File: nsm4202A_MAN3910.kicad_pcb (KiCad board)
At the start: 2 copper layers, 40.5 x 25.5 mm, 19 parts, among them IC1 IS31FL3730-QFLS2-TR, IC2 IS31FL3730-QFLS2-TR, J1 Conn_01x07_Pin, J2 Conn_01x02_Pin, J3 Conn_01x03_Pin

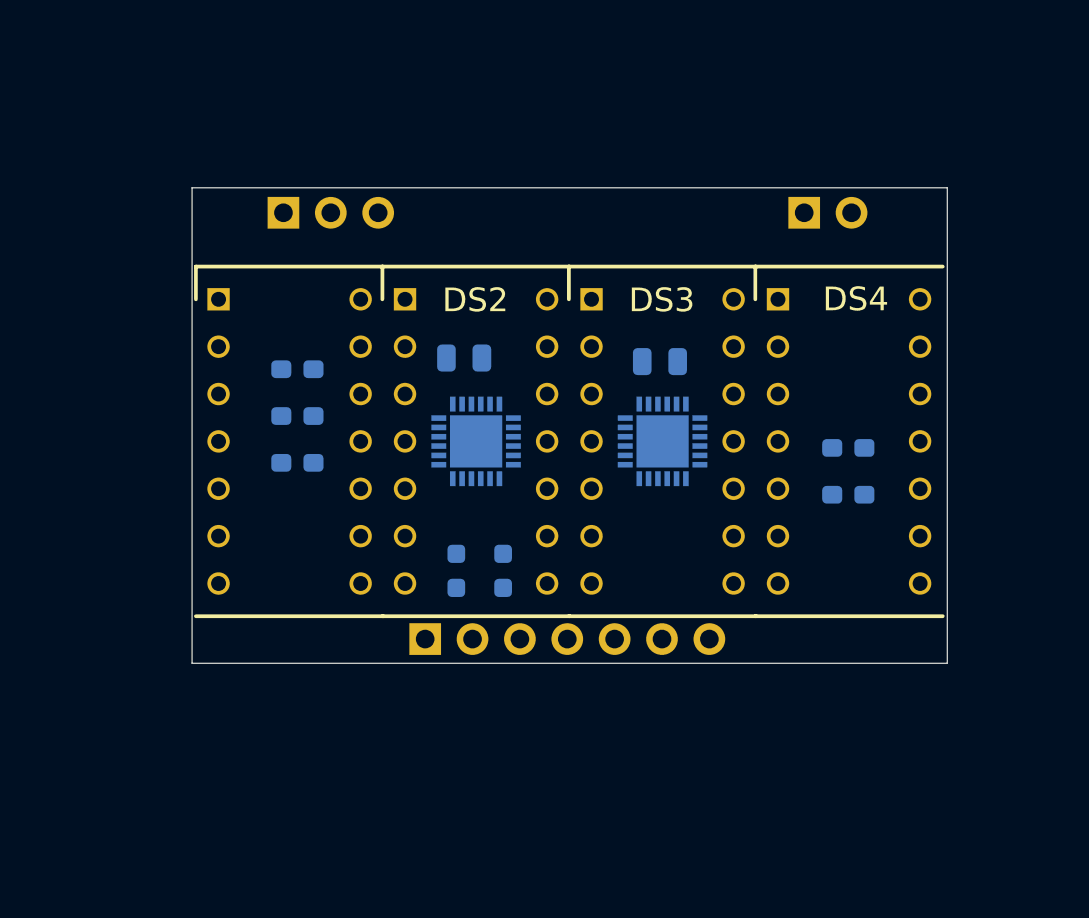
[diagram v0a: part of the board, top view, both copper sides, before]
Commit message: Start trace
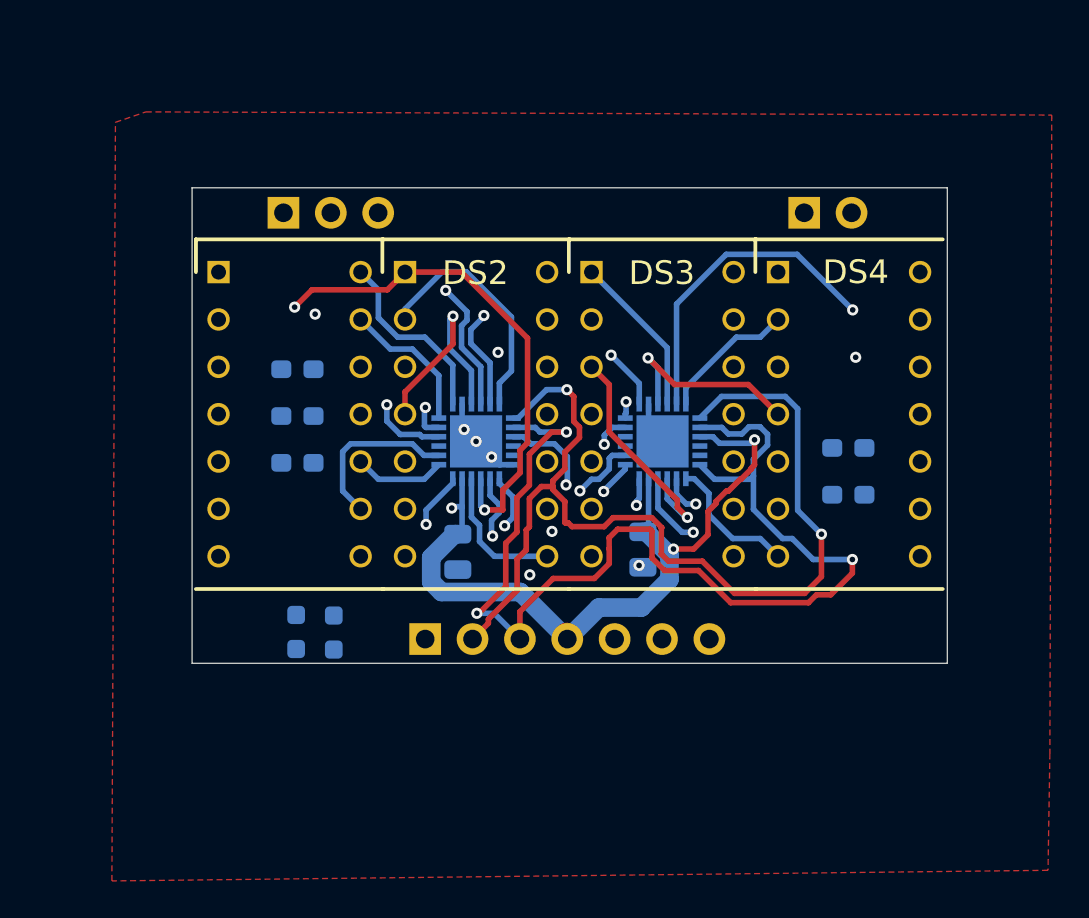
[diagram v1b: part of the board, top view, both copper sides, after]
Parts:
- moved R2 11.6 mm to (105.6, 98.8)
- moved C3 10.4 mm to (114.2, 94.5), turned to -90 degrees
- moved C7 10.1 mm to (124.2, 94.4), turned to -90 degrees
- moved R1 7.36 mm to (107.6, 98.8)
- moved DS1 1.46 mm to (101.4, 79.5)
- moved DS2 1.46 mm to (111.4, 79.5)
- moved DS3 1.46 mm to (121.4, 79.5)
- moved DS4 1.46 mm to (131.4, 79.5)
- turned IC1 to 180 degrees
- turned IC2 to 180 degrees
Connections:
- IC1 pad 1: Net-(IC1-SDA) -> /SDA
- IC1 pad 2: Net-(IC1-SCL) -> /SCL
- IC2 pad 1: unconnected-(IC2-SDA-Pad1) -> /SDA
- IC2 pad 2: Net-(IC2-AD) -> /SCL
- IC2 pad 6: Net-(IC2-AD) -> /SCL
- J1 pad 2: unconnected-(J1-Pin_2-Pad2) -> /SDA
- J1 pad 3: unconnected-(J1-Pin_3-Pad3) -> /SCL
- J1 pad 4: unconnected-(J1-Pin_4-Pad4) -> +5V
- J1 pad 6: unconnected-(J1-Pin_6-Pad6) -> GND
- J1 pad 7: unconnected-(J1-Pin_7-Pad7) -> /D1_C8
- J2 pad 1: unconnected-(J2-Pin_1-Pad1) -> /D1_R4
- J2 pad 2: unconnected-(J2-Pin_2-Pad2) -> /D1_R5
- J3 pad 1: unconnected-(J3-Pin_1-Pad1) -> /D1_R1
- J3 pad 2: unconnected-(J3-Pin_2-Pad2) -> /D1_R2
- J3 pad 3: unconnected-(J3-Pin_3-Pad3) -> /D1_R3
- R1 pad 2: Net-(IC1-SCL) -> /SCL
- R2 pad 2: Net-(IC1-SDA) -> /SDA
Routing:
- net /SCL: track 0.00 -> 62.0 mm, vias 0 -> 3
- net +5V: track 0.00 -> 59.5 mm, vias 0 -> 6
- net /SDA: track 0.00 -> 54.7 mm, vias 0 -> 2
- net /D2_C2: track 0.00 -> 46.8 mm, vias 0 -> 1
- net /D1_R4: track 0.00 -> 43.5 mm
- net /D1_R5: track 0.00 -> 43.5 mm, vias 0 -> 1
- net /D2_R1: track 0.00 -> 42.9 mm
- net /D1_R3: track 0.00 -> 36.4 mm, vias 0 -> 2
- net /D2_C6: track 0.00 -> 34.6 mm, vias 0 -> 1
- net /D1_R1: track 0.00 -> 34.5 mm, vias 0 -> 1
- net /D1_R6: track 0.00 -> 33.9 mm, vias 0 -> 1
- net /D2_R4: track 0.00 -> 33.5 mm, vias 0 -> 1
- net /D1_C3: track 0.00 -> 33.0 mm, vias 0 -> 1
- net /D1_C5: track 0.00 -> 32.8 mm
- net /D1_C2: track 0.00 -> 32.3 mm, vias 0 -> 2
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- added copper zone on F.Cu, net GND
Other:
- copper layers 2 -> 4
